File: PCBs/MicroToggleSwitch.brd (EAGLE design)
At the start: 14.5 x 31.7 mm, 3 parts

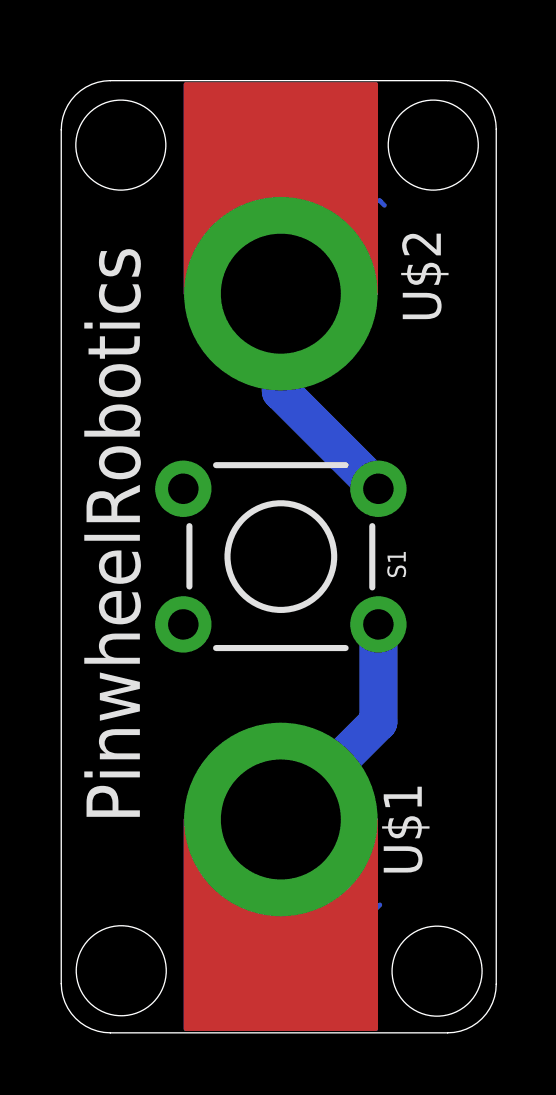
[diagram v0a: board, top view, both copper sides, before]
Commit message: New Update
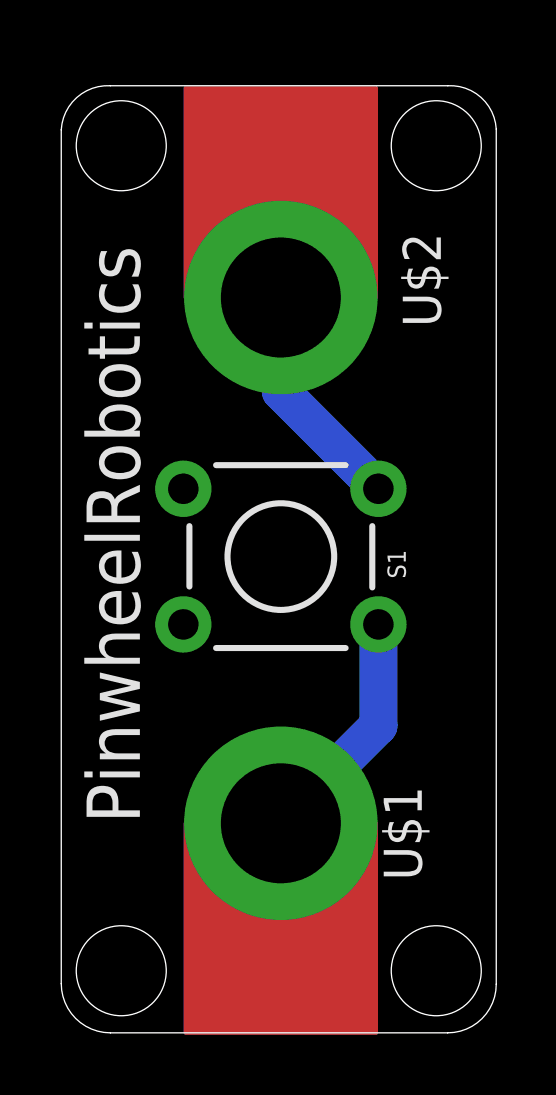
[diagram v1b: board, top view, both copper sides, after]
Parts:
- moved U$1 0.13 mm to (20.3, 18.4)
- moved U$2 0.13 mm to (20.3, 35.9)
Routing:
- net N$2: track 14.4 -> 7.77 mm
- net N$1: track 14.4 -> 8.05 mm
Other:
- board size 14.5 x 31.7 mm -> 14.5 x 31.6 mm
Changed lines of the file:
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@@
 <drawing>
 <settings>
-<setting alwaysvectorfont="yes"/>
+<setting alwaysvectorfont="no"/>
 <setting verticaltext="up"/>
 </settings>
@@
 <wire x1="25.88049375" y1="11.43" x2="27.5" y2="13.04950625" width="0" layer="20" curve="90"/>
 <wire x1="27.5" y1="13.04950625" x2="27.5" y2="41.55424375" width="0" layer="20"/>
-<wire x1="27.5" y1="41.55424375" x2="25.88424375" y2="43.17" width="0" layer="20" curve="90"/>
-<wire x1="25.88424375" y1="43.17" x2="14.638371875" y2="43.17" width="0" layer="20"/>
-<wire x1="14.638371875" y1="43.17" x2="13" y2="41.531628125" width="0" layer="20" curve="90"/>
-<hole x="14.986" y="41.021" drill="3"/>
-<hole x="25.4" y="41.021" drill="3"/>
+<wire x1="27.5" y1="41.55424375" x2="25.88424375" y2="43" width="0" layer="20" curve="90"/>
+<wire x1="25.88424375" y1="43" x2="14.638371875" y2="43" width="0" layer="20"/>
+<wire x1="14.638371875" y1="43" x2="13" y2="41.531628125" width="0" layer="20" curve="90"/>
+<hole x="15" y="41" drill="3"/>
+<hole x="25.5" y="41" drill="3"/>
 <hole x="15" y="13.5" drill="3"/>
-<hole x="25.527" y="13.486" drill="3"/>
+<hole x="25.5" y="13.5" drill="3"/>
 <text x="15.621" y="18.415" size="1.778" layer="21" rot="R90">PinwheelRobotics </text>
 <text x="27.051" y="36.957" size="1.778" layer="22" rot="MR270">care@pinwheel.in</text>
@@
 <attribute name="SF_SKU" value="COM-00097" x="-1.27" y="62.865" size="1.778" layer="27" rot="R180" display="off"/>
 </element>
-<element name="U$1" library="microbit" package="MICROBIT_PAD" value="MICROBIT_PAD" x="20.32" y="18.542" smashed="yes">
-<attribute name="NAME" x="25.019" y="16.637" size="1.27" layer="21" rot="R90"/>
+<element name="U$1" library="microbit" package="MICROBIT_PAD" value="MICROBIT_PAD" x="20.32" y="18.415" smashed="yes">
+<attribute name="NAME" x="25.019" y="16.51" size="1.27" layer="21" rot="R90"/>
 </element>
-<element name="U$2" library="microbit" package="MICROBIT_PAD" value="MICROBIT_PAD" x="20.32" y="36.068" smashed="yes" rot="R180">
-<attribute name="NAME" x="24.384" y="38.227" size="1.27" layer="21" rot="R270"/>
+<element name="U$2" library="microbit" package="MICROBIT_PAD" value="MICROBIT_PAD" x="20.32" y="35.941" smashed="yes" rot="R180">
+<attribute name="NAME" x="24.384" y="38.1" size="1.27" layer="21" rot="R270"/>
 </element>
 </elements>
@@
 <contactref element="U$1" pad="PAD"/>
 <contactref element="S1" pad="1"/>
-<wire x1="23.3172" y1="15.3924" x2="23.622" y2="15.6972" width="0.1524" layer="16"/>
-<wire x1="20.4216" y1="15.3924" x2="23.3172" y2="15.3924" width="0.1524" layer="16"/>
-<wire x1="20.32" y1="18.542" x2="20.4216" y2="15.3924" width="0.1524" layer="16"/>
 <wire x1="23.622" y1="24.9936" x2="23.5712" y2="25.0444" width="0.1524" layer="16"/>
-<wire x1="23.5712" y1="25.0444" x2="23.5712" y2="21.7932" width="1.27" layer="16"/>
-<wire x1="23.5712" y1="21.7932" x2="20.32" y2="18.542" width="1.27" layer="16"/>
+<wire x1="23.5712" y1="25.0444" x2="23.5712" y2="21.6662" width="1.27" layer="16"/>
+<wire x1="23.5712" y1="21.6662" x2="20.32" y2="18.415" width="1.27" layer="16"/>
 </signal>
 <signal name="N$2">
 <contactref element="U$2" pad="PAD"/>
 <contactref element="S1" pad="3"/>
-<wire x1="23.622" y1="39.1668" x2="23.7744" y2="39.0144" width="0.1524" layer="16"/>
-<wire x1="20.574" y1="39.1668" x2="23.622" y2="39.1668" width="0.1524" layer="16"/>
-<wire x1="20.2692" y1="38.862" x2="20.574" y2="39.1668" width="0.1524" layer="16"/>
 <wire x1="23.622" y1="29.5656" x2="23.5712" y2="29.5656" width="0.1524" layer="16"/>
-<wire x1="20.2692" y1="38.862" x2="20.32" y2="36.068" width="0.1524" layer="16"/>
 <wire x1="23.5712" y1="29.5656" x2="20.32" y2="32.8168" width="1.27" layer="16"/>
-<wire x1="20.32" y1="32.8168" x2="20.32" y2="36.068" width="1.27" layer="16"/>
+<wire x1="20.32" y1="32.8168" x2="20.32" y2="35.941" width="1.27" layer="16"/>
 </signal>
 </signals>
